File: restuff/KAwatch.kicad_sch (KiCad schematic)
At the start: 22 parts, among them J1 Conn_01x08, J2 USB_C_Receptacle_PowerOnly_6P, J3 Conn_01x02, J4 Conn_01x02, Q1 Q_NPN_BCE, SW1 SW_Push, U1 ESP32-WROOM-32E, U2 MCP73831-2-OT, U3 AMS1117-3.3

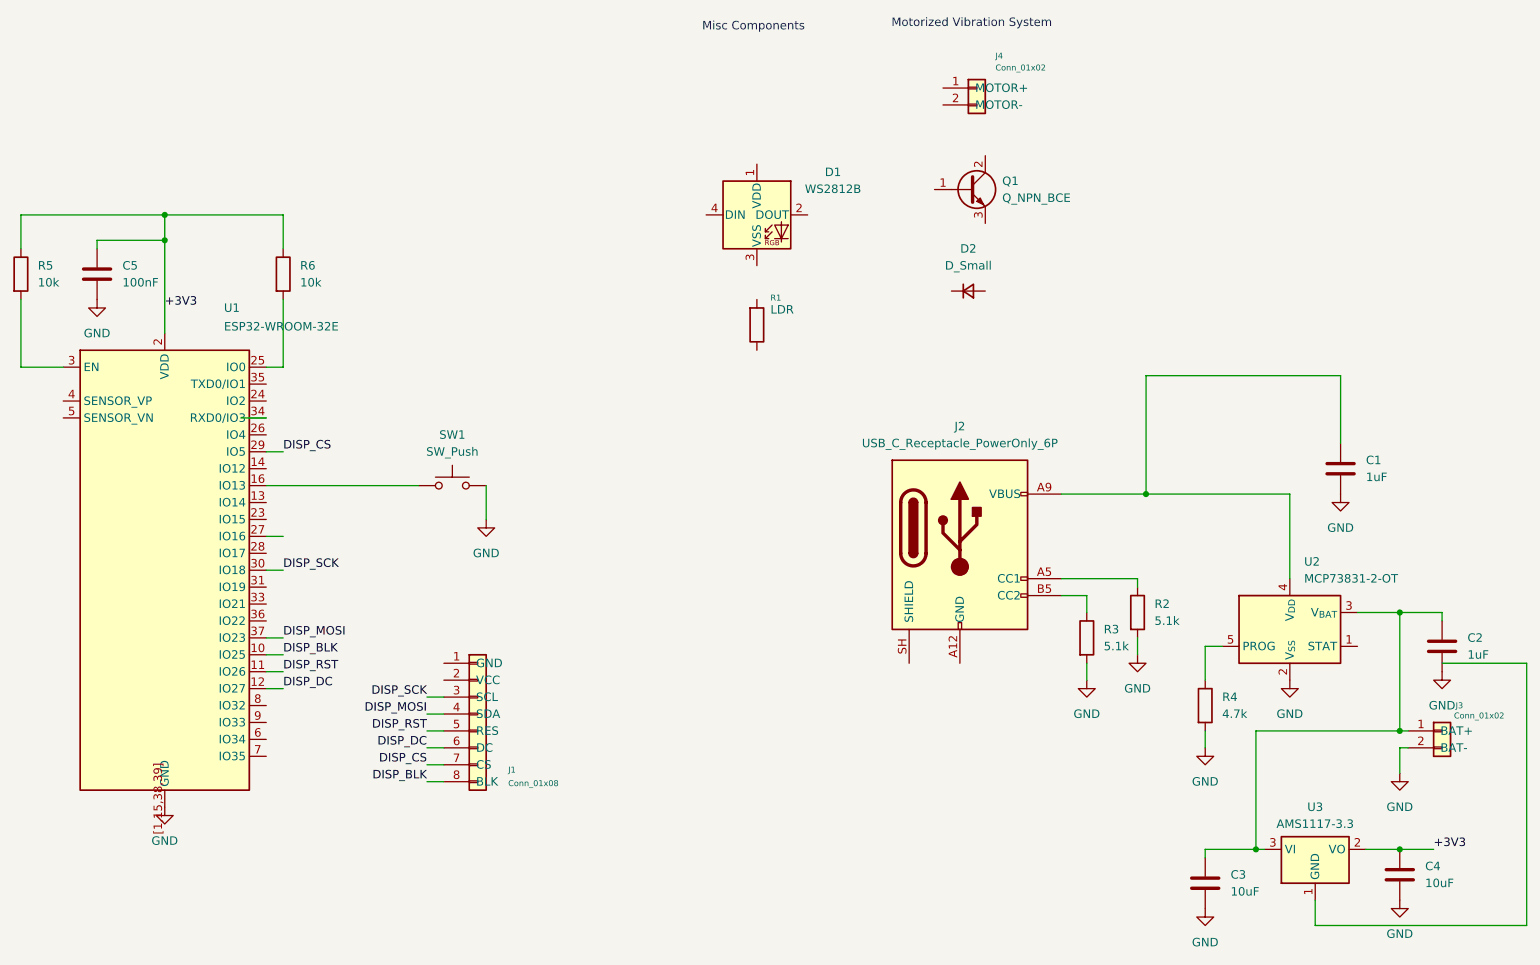
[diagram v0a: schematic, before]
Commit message: motor components added
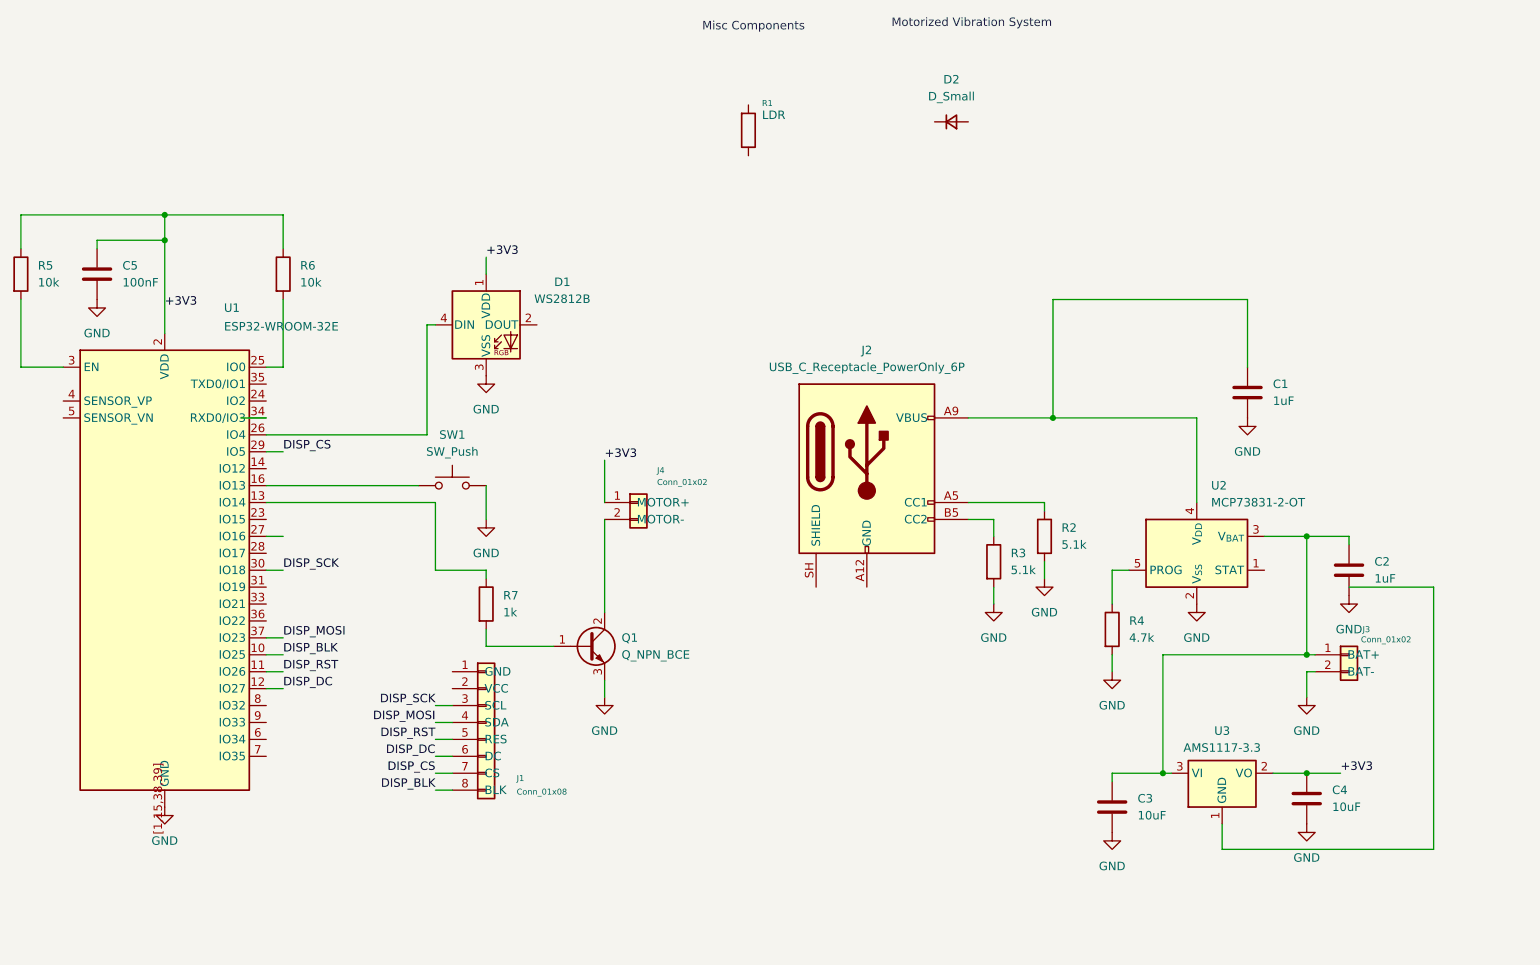
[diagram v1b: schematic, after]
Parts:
- added R7: 1k, symbol Device:R
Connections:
- net +3V3: now also D1.1 (VDD), J4.1 (MOTOR+)
- net GND: now also D1.3 (VSS), Q1.3 (E)
- net at J4.2 (MOTOR-): now also Q1.2 (C)
- net at Q1.1 (B): now also R7.2
- net at D1.4 (DIN): now also U1.26 (IO4)
- net at U1.13 (IO14): now also R7.1
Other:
- moved on the sheet: C1, C2, C3, C4, D1, D2, J1, J2, J3, J4, Q1, R1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
